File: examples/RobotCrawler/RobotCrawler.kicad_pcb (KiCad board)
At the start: 2 copper layers, 50 x 50 mm, 52 parts

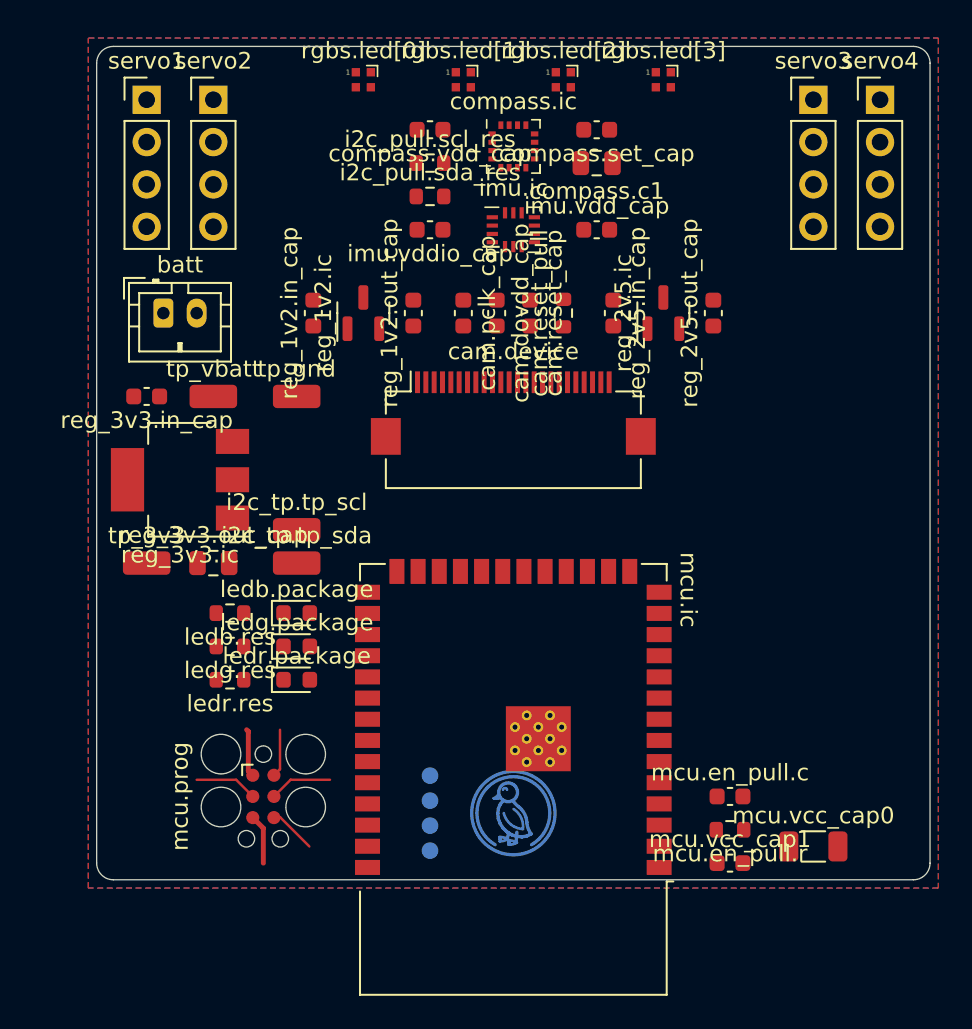
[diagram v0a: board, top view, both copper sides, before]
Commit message: layout round 2
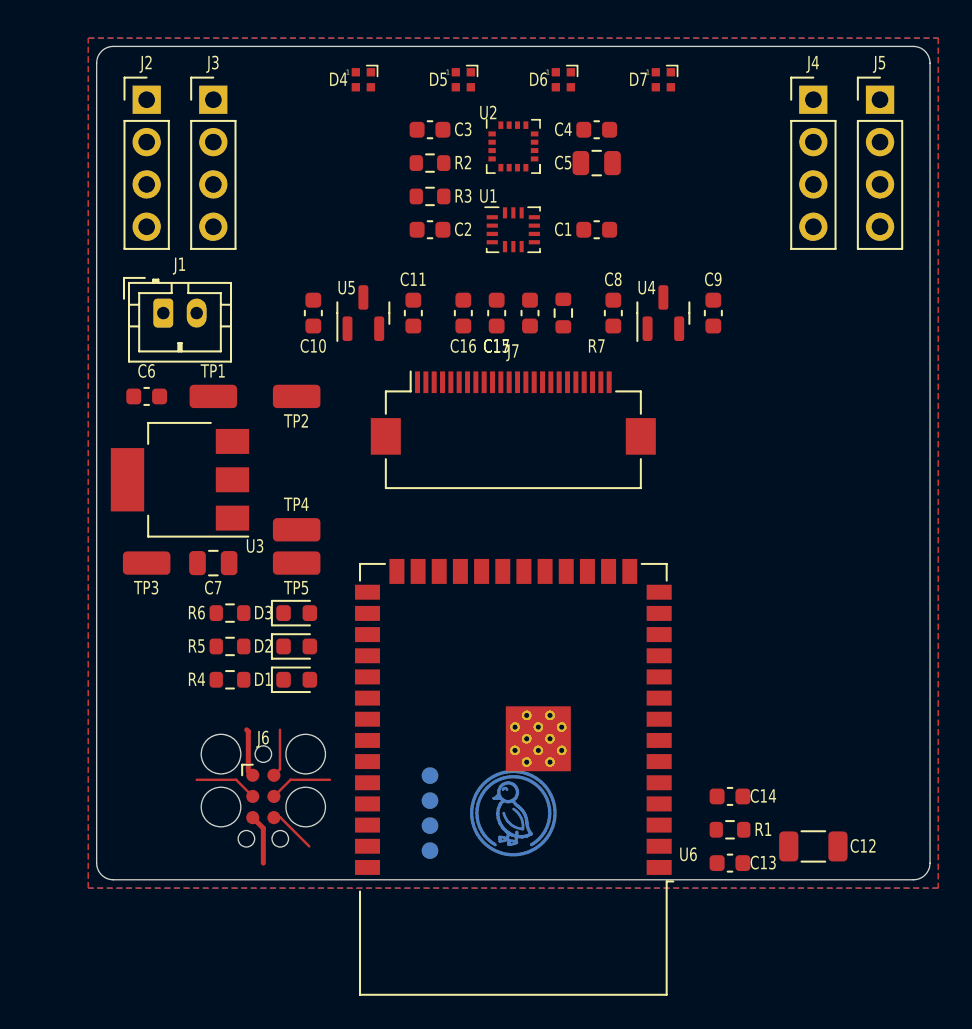
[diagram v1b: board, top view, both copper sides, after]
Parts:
- turned C10 to -90 degrees
- turned C15 to 90 degrees
- turned C16 to 90 degrees
- turned C17 to 90 degrees
- turned R7 to -90 degrees
- renumbered imu.vdd_cap to C1, reg_1v2.in_cap to C10, reg_1v2.out_cap to C11, mcu.vcc_cap0 to C12, mcu.vcc_cap1 to C13, mcu.en_pull.c to C14, cam.dovdd_cap to C15, cam.pclk_cap to C16, cam.reset_cap to C17, imu.vddio_cap to C2, compass.vdd_cap to C3, compass.set_cap to C4, compass.c1 to C5, reg_3v3.in_cap to C6, reg_3v3.out_cap to C7, reg_2v5.in_cap to C8, reg_2v5.out_cap to C9, ledr.package to D1, ledg.package to D2, ledb.package to D3, rgbs.led[0] to D4, rgbs.led[1] to D5, rgbs.led[2] to D6, rgbs.led[3] to D7, batt to J1, servo1 to J2, servo2 to J3, servo3 to J4, servo4 to J5, mcu.prog to J6, cam.device to J7, mcu.en_pull.r to R1, i2c_pull.scl_res to R2, i2c_pull.sda_res to R3, ledr.res to R4, ledg.res to R5, ledb.res to R6, cam.reset_pull to R7, tp_vbatt to TP1, tp_gnd to TP2, tp_3v3 to TP3, i2c_tp.tp_scl to TP4, i2c_tp.tp_sda to TP5, imu.ic to U1, compass.ic to U2, reg_3v3.ic to U3, reg_2v5.ic to U4, reg_1v2.ic to U5, mcu.ic to U6
